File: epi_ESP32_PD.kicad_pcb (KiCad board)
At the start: 4 copper layers, 22.7 x 54.9 mm, 66 parts, among them J1 Conn_01x08, J2 USB_C_Receptacle_USB2.0, J3 Conn_01x08, J4 Conn_01x01, J6 Conn_Coaxial_Small, J7 Conn_02x03, J8 Conn_01x03, Q1 Q_PMOS_GDS, Q2 Q_NMOS_GDS, Q3 Q_NMOS_GDS, Q4 Q_NMOS_GDS, Q5 Q_NMOS_GDS, Q6 Q_NMOS_GDS, SW1 SW_MEC_5G, SW2 SW_MEC_5G, U1 ESP32-C3, U2 MIC5219-3.3YM5, U5 AP63205WU, Y1 Crystal

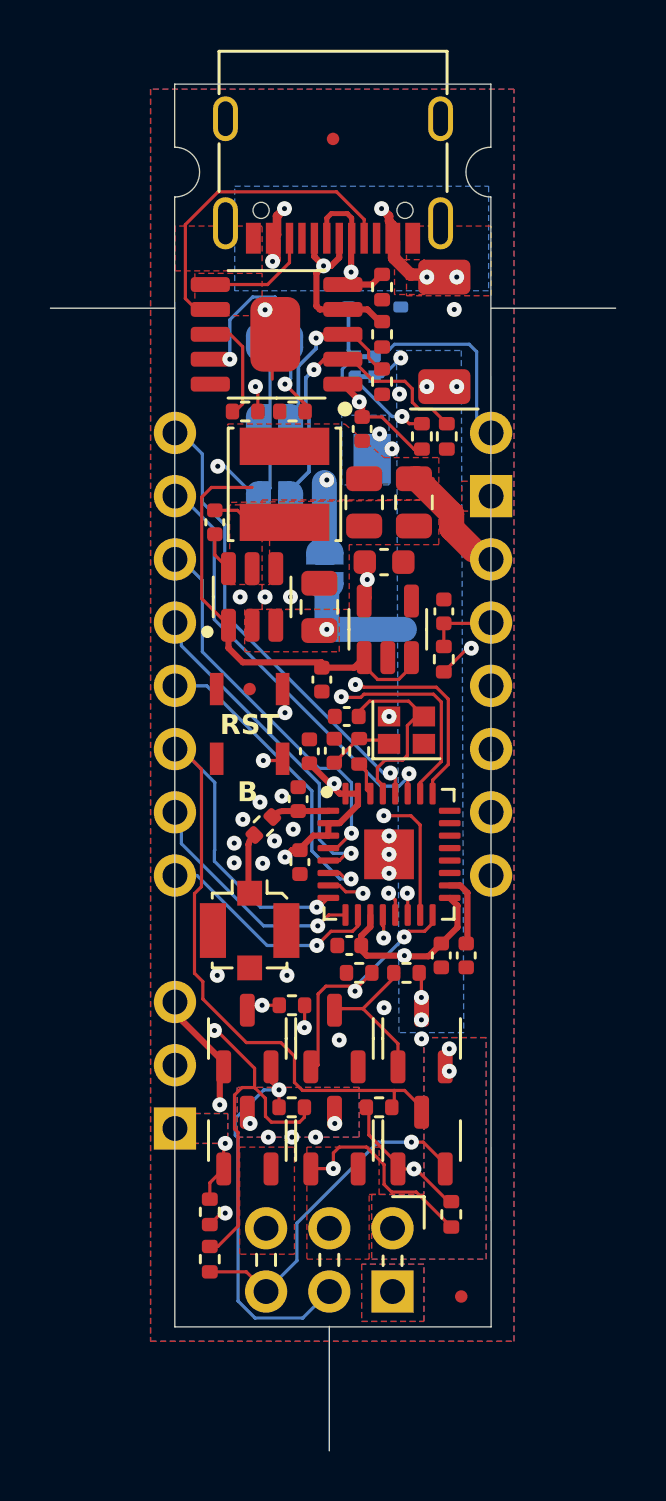
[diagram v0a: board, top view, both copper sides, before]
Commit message: revision
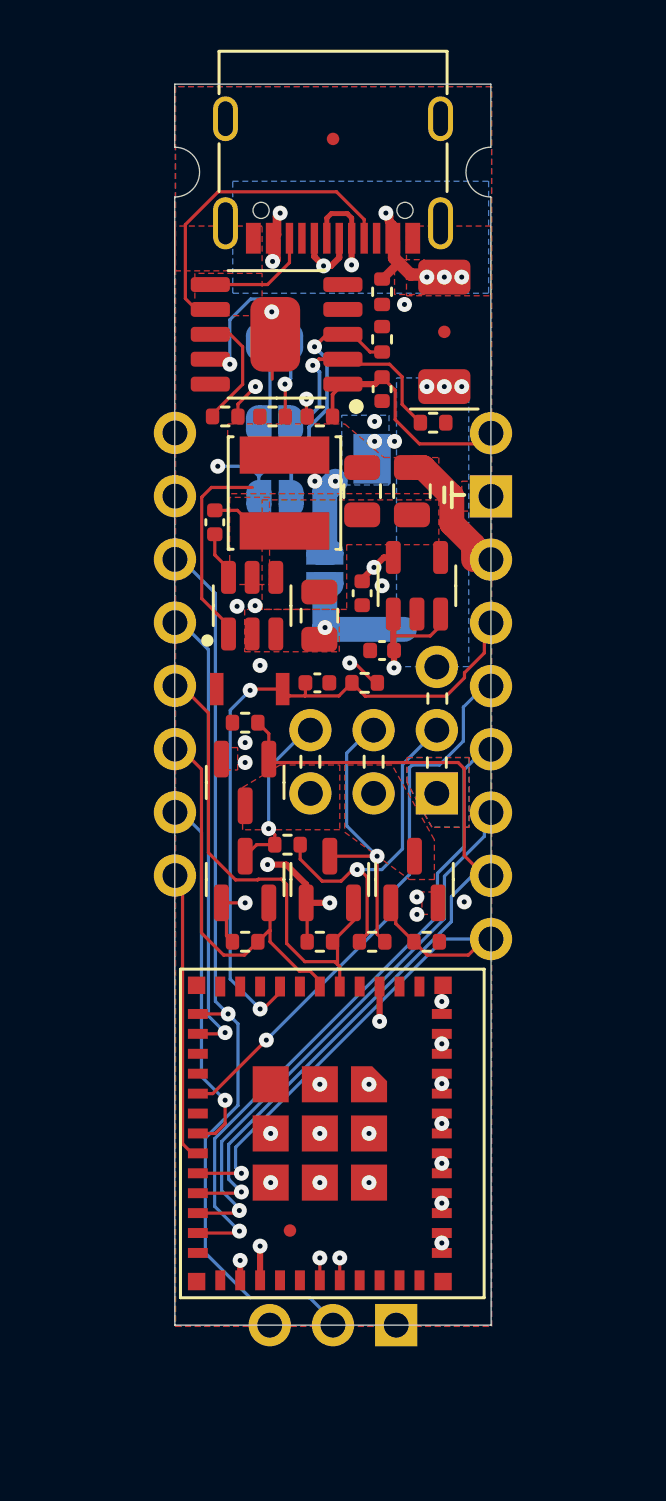
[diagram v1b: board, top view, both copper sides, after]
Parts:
- removed C12, C5: 1µF, Capacitor_SMD:C_0402_1005Metric
- removed C14: 22µF, Capacitor_SMD:C_0603_1608Metric
- removed C2, C7: 100nF, Capacitor_SMD:C_0402_1005Metric
- removed C3, C4, C6: TBD, Capacitor_SMD:C_0402_1005Metric
- removed D2: D_Zener, Diode_SMD:D_SOD-323
- removed J3: Conn_01x08, Connector_PinHeader_2.54mm:PinHeader_1x08_P2.54mm_Vertical
- removed J6: Conn_Coaxial_Small, Connector_Coaxial:U.FL_Molex_MCRF_73412-0110_Vertical
- removed JP5, JP6: Jumper, Jumper:SolderJumper-2_P1.3mm_Bridged_RoundedPad1.0x1.5mm
- removed L1: TBD, Resistor_SMD:R_0402_1005Metric
- removed Q5, Q6: Q_NMOS_GDS, Package_TO_SOT_SMD:SOT-23-3
- removed R2: 22Ω, Resistor_SMD:R_0402_1005Metric
- removed R4, R5: 10K, Resistor_SMD:R_0402_1005Metric
- removed RV2: Varistor, Resistor_SMD:R_0402_1005Metric
- removed SW1: SW_MEC_5G, DIY:R-668048
- removed Y1: Crystal, Crystal:Crystal_SMD_2016-4Pin_2.0x1.6mm
- added J5: Conn_01x09, Connector_PinHeader_2.54mm:PinHeader_1x09_P2.54mm_Vertical, F.Cu at (106.7, 48.3)
- C1: value 100nF -> 1µF
- Q1: value Q_PMOS_GDS -> Q_NMOS_GSD; footprint Package_TO_SOT_SMD:SOT-23-3 -> Package_TO_SOT_SMD:SOT-23
- Q2, Q3, Q4: value Q_NMOS_GDS -> Q_NMOS_GSD; footprint Package_TO_SOT_SMD:SOT-23-3 -> Package_TO_SOT_SMD:SOT-23
- R1: value 1K -> TBD
- R15, R3, R8: value 10K -> 1K
- U1: value ESP32-C3 -> ESP32-C3-MINI-1; footprint Package_DFN_QFN:QFN-32-1EP_5x5mm_P0.5mm_EP3.45x3.45mm -> PCM_Espressif:ESP32-C3-MINI-1
- moved J7 20.1 mm to (104.5, 60.2)
- moved R14 19.7 mm to (96.8, 59.9), turned to 0 degrees
- moved R12 16.9 mm to (98.5, 64.8), turned to 0 degrees
- moved REF** 16.3 mm to (104.8, 44.2)
- moved C1 14.9 mm to (101.5, 54.7)
- moved J8 13.5 mm to (97.8, 84.1), turned to 90 degrees
- moved U1 11.2 mm to (102.5, 76.4), turned to -90 degrees
- moved Q2 11.1 mm to (96.8, 66.2)
- moved R13 11.0 mm to (104.1, 68.7), turned to 180 degrees
- moved Q4 10.5 mm to (103.6, 66.2)
- moved Q3 10.3 mm to (96.8, 62.3), turned to -90 degrees
- moved R11 8.55 mm to (96.8, 68.7)
- moved R10 7.39 mm to (101.9, 68.7), turned to 180 degrees
- moved Q1 7.38 mm to (100.2, 66.2)
- moved REF** 7.37 mm to (98.6, 80.3)
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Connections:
- C8 pad 1: Net-(D2-K) -> +3.3V
- D1 pad 2: /PD -> PD
- J2 pad A4: /PD -> PD
- J2 pad A9: /PD -> PD
- J2 pad B4: /PD -> PD
- J2 pad B9: /PD -> PD
- J7 pad 1: VOUT -> +5V
- J7 pad 3: B -> IO2_5V
- J7 pad 4: IO2_5V -> B
- J7 pad 5: W -> IO3_5V
- J7 pad 6: IO3_5V -> W
- Q1 pad 1: Net-(Q1-G) -> +3.3V
- Q1 pad 2: VOUT -> IO2
- Q1 pad 3: VIN -> IO2_5V
- Q2 pad 1: IO6 -> +3.3V
- Q2 pad 2: B -> IO3
- Q2 pad 3: GND -> IO3_5V
- Q3 pad 1: +3.3V -> IO7
- Q3 pad 2: IO2_5V -> GND
- Q3 pad 3: IO2 -> W
- Q4 pad 1: +3.3V -> IO6
- Q4 pad 2: IO3_5V -> GND
- Q4 pad 3: IO3 -> B
- R1 pad 1: Net-(D2-K) -> +3.3V
- R1 pad 2: Net-(JP5-A) -> PD
- R13 pad 1: IO6 -> GND
- R13 pad 2: +3.3V -> IO6
- R14 pad 1: IO7 -> GND
- R14 pad 2: +3.3V -> IO7
- R7 pad 1: /PD -> PD
- RV3 pad 1: D- -> PD
- U1 pad 1: Net-(U1-LNA_IN) -> GND
- U1 pad 10: IO5 -> unconnected-(U1-NC-Pad10)
- U1 pad 11: +3.3V -> GND
- U1 pad 12: IO6 -> IO0
- U1 pad 13: IO7 -> IO1
- U1 pad 14: IO8 -> GND
- U1 pad 15: BOOT -> unconnected-(U1-NC-Pad15)
- U1 pad 17: +3.3V -> unconnected-(U1-NC-Pad17)
- U1 pad 18: Net-(U1-VDD_SPI/GPIO11) -> IO4
- U1 pad 19: unconnected-(U1-SPIHD/GPIO12-Pad19) -> IO5
- U1 pad 2: +3.3V -> GND
- U1 pad 20: unconnected-(U1-SPIWP/GPIO13-Pad20) -> IO6
- U1 pad 21: unconnected-(U1-SPICS0/GPIO14-Pad21) -> IO7
- U1 pad 22: unconnected-(U1-SPICLK/GPIO15-Pad22) -> IO8
- U1 pad 23: unconnected-(U1-SPID/GPIO16-Pad23) -> BOOT
- U1 pad 25: D- -> unconnected-(U1-NC-Pad25)
- U1 pad 26: D+ -> D-
- U1 pad 27: U0RXD -> D+
- U1 pad 28: U0TXD -> unconnected-(U1-NC-Pad28)
- U1 pad 29: Net-(U1-XTAL_N) -> unconnected-(U1-NC-Pad29)
- U1 pad 30: Net-(U1-XTAL_P) -> U0RXD
- U1 pad 31: +3.3V -> U0TXD
- U1 pad 32: +3.3V -> unconnected-(U1-NC-Pad32)
- U1 pad 33: GND -> unconnected-(U1-NC-Pad33)
- U1 pad 4: IO0 -> unconnected-(U1-NC-Pad4)
- U1 pad 5: IO1 -> IO2
- U1 pad 6: IO2 -> IO3
- U1 pad 7: EN -> unconnected-(U1-NC-Pad7)
- U1 pad 8: IO3 -> EN
- U1 pad 9: IO4 -> unconnected-(U1-NC-Pad9)
- U3 pad 1: Net-(D2-K) -> +3.3V
- U3 pad 4: D+ -> unconnected-(U3-DP-Pad4)
- U3 pad 5: D- -> unconnected-(U3-DM-Pad5)
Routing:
- net +5V: track 63.7 -> 35.5 mm, vias 2 -> 4
- net U0TXD: track 18.2 -> 40.4 mm
- net U0RXD: track 17.2 -> 37.5 mm
- net /PD: track 18.0 -> 0.00 mm, vias 7 -> 0
- net D-: track 30.9 -> 48.8 mm
- net IO3: track 33.6 -> 15.7 mm, vias 1 -> 0
- net +3.3V: track 46.6 -> 30.0 mm, vias 10 -> 7
- net PD: track 0.00 -> 16.3 mm, vias 0 -> 8
- net IO8: track 7.96 -> 22.4 mm
- net D+: track 33.2 -> 46.8 mm
- net IO10: track 10.1 -> 22.1 mm, vias 2 -> 1
- net IO7: track 22.7 -> 33.5 mm, vias 2 -> 1
- net Net-(D2-K): track 9.18 -> 0.00 mm, vias 1 -> 0
- net Net-(U1-XTAL_N): track 7.49 -> 0.00 mm
- net IO0: track 29.6 -> 36.8 mm
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- added copper zone on In2.Cu, net +5V
- added copper zone on B.Cu, net PD
- added copper zone on F.Cu, net PD
- added copper zone on In2.Cu, net PD
- removed copper zone on B.Cu, net /PD
- removed copper zone on F.Cu, net /PD
- removed copper zone on In2.Cu, net /PD
- removed copper zone on B.Cu, net VOUT
- removed copper zone on F.Cu, net VOUT
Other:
- board size 22.7 x 54.9 mm -> 12.7 x 49.8 mm
- board text added: "Epi-C3-PD V1,1"
- board text added: "IO2-5"
- board text added: "IO3-5"
- board text added: "R"
- board text removed: "8"
- board text removed: "BOOT"
- board text removed: "Epi-C3-PD"
- board text removed: "IO2-5V"
- board text removed: "IO3-5V"
- board text removed: "RST"
- board text removed: "VOUT"
